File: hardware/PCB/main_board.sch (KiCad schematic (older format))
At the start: 0 parts

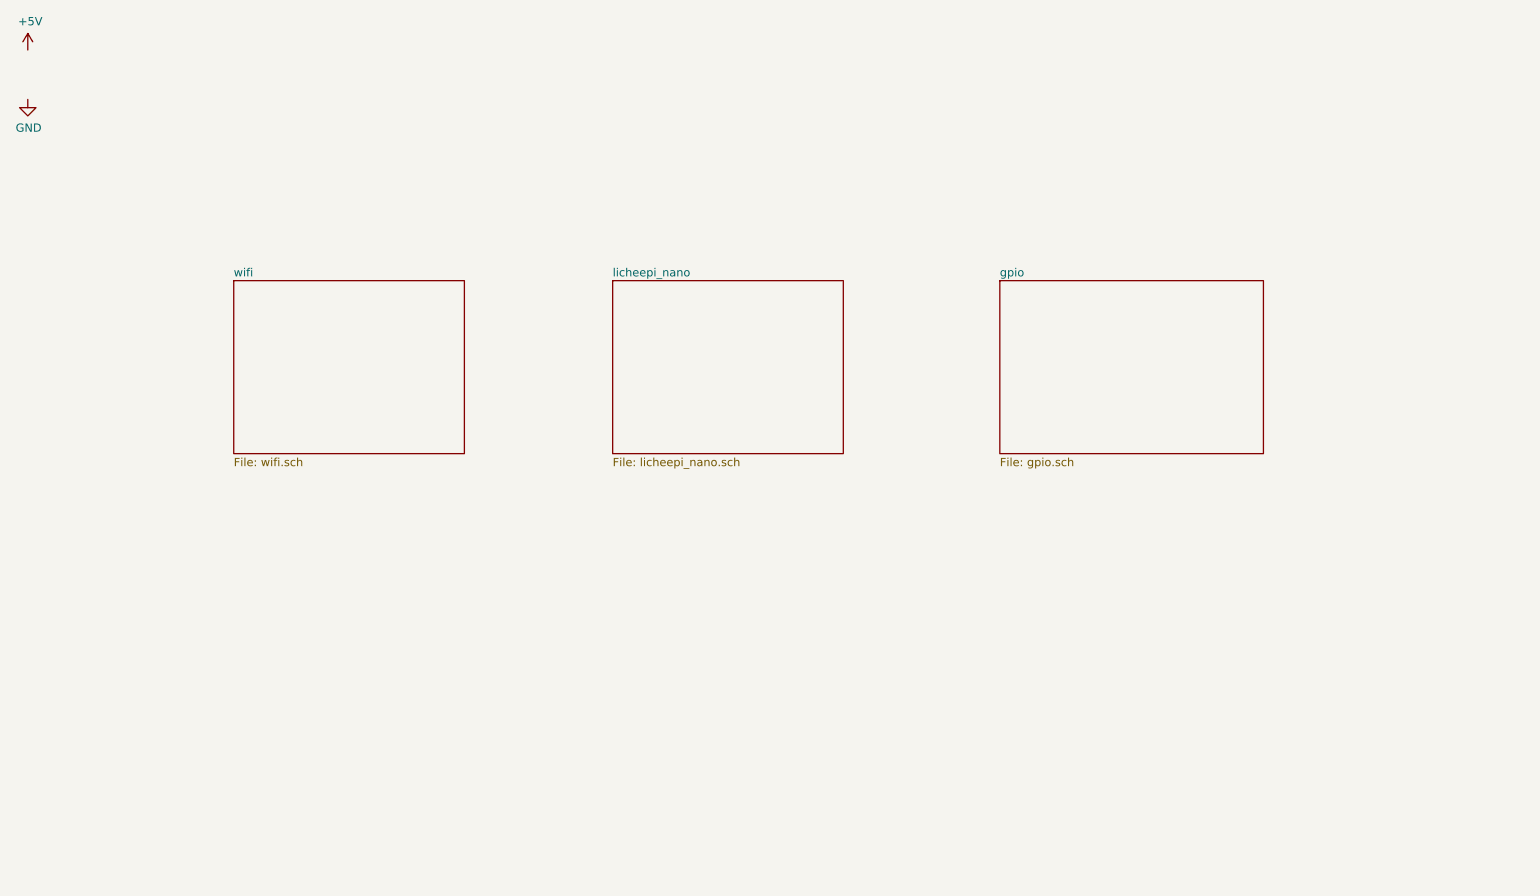
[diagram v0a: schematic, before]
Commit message: update pcb,
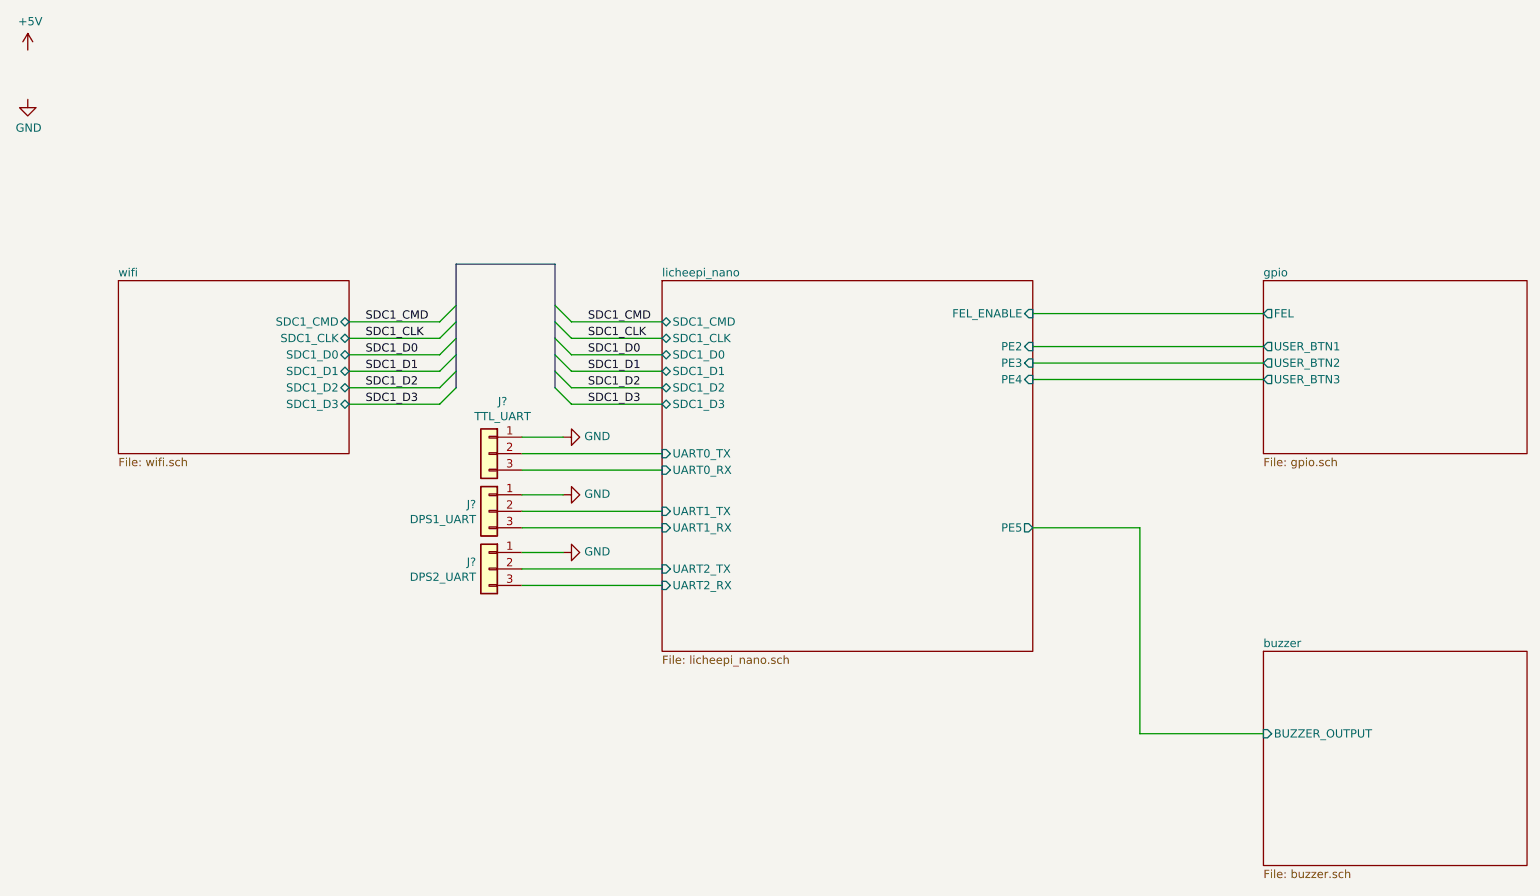
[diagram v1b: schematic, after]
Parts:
- added J?: TTL_UART, symbol Connector_Generic:Conn_01x03
- added J?: DPS1_UART, symbol Connector_Generic:Conn_01x03
- added J?: DPS2_UART, symbol Connector_Generic:Conn_01x03
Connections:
- net GND: now also J?.1 (Pin_1), J?.1 (Pin_1), J?.1 (Pin_1)
- new net licheepi_nano/UART0_RX: J?.3 (Pin_3)
- new net licheepi_nano/UART0_TX: J?.2 (Pin_2)
- new net licheepi_nano/UART1_RX: J?.3 (Pin_3)
- new net licheepi_nano/UART1_TX: J?.2 (Pin_2)
- new net licheepi_nano/UART2_RX: J?.3 (Pin_3)
- new net licheepi_nano/UART2_TX: J?.2 (Pin_2)
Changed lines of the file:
@@
 $Descr A4 11693 8268
 encoding utf-8
-Sheet 1 4
+Sheet 1 5
 Title ""
 Date ""
@@
 $EndDescr
 $Comp
-L customized_power:+5V #PWR?
+L customized_power:+5V #PWR0101
 U 1 1 5E8767E8
 P 950 1000
-F 0 "#PWR?" H 950 850 50  0001 C CNN
+F 0 "#PWR0101" H 950 850 50  0001 C CNN
 F 1 "+5V" H 965 1173 50  0000 C CNN
 F 2 "" H 950 1000 50  0001 C CNN
@@
 $EndComp
 $Comp
-L power:GND #PWR?
+L power:GND #PWR0102
 U 1 1 5E876DA9
 P 950 1300
-F 0 "#PWR?" H 950 1050 50  0001 C CNN
+F 0 "#PWR0102" H 950 1050 50  0001 C CNN
 F 1 "GND" H 955 1127 50  0000 C CNN
 F 2 "" H 950 1300 50  0001 C CNN
@@
 	1    0    0    -1
 $EndComp
-$Sheet
-S 4500 2400 1400 1050
+Entry Wire Line
+	3450 3150 3550 3050
+Entry Wire Line
+	3450 3050 3550 2950
+Entry Wire Line
+	3450 2950 3550 2850
+Entry Wire Line
+	3450 2850 3550 2750
+Entry Wire Line
+	3450 2750 3550 2650
+Entry Wire Line
+	3450 2650 3550 2550
+Wire Bus Line
+	3550 2300 4150 2300
+Entry Wire Line
+	4150 2550 4250 2650
+Entry Wire Line
+	4150 2650 4250 2750
+Entry Wire Line
+	4150 2750 4250 2850
+Entry Wire Line
+	4150 2850 4250 2950
+Entry Wire Line
+	4150 2950 4250 3050
+Entry Wire Line
+	4150 3050 4250 3150
+Wire Wire Line
+	4250 2650 4800 2650
+Wire Wire Line
+	4250 2750 4800 2750
+Wire Wire Line
+	4250 2850 4800 2850
+Wire Wire Line
+	4250 2950 4800 2950
+Wire Wire Line
+	4250 3050 4800 3050
+Wire Wire Line
+	4250 3150 4800 3150
+Wire Wire Line
+	2900 3150 3450 3150
+Wire Wire Line
+	2900 2650 3450 2650
+Wire Wire Line
+	2900 2750 3450 2750
+Wire Wire Line
+	2900 2850 3450 2850
+Wire Wire Line
+	2900 2950 3450 2950
+Wire Wire Line
+	2900 3050 3450 3050
+$Sheet
+S 1500 2400 1400 1050
+U 5E8B2717
+F0 "wifi" 50
+F1 "wifi.sch" 50
+F2 "SDC1_D2" B R 2900 3050 50
+F3 "SDC1_D1" B R 2900 2950 50
+F4 "SDC1_D0" B R 2900 2850 50
+F5 "SDC1_CLK" B R 2900 2750 50
+F6 "SDC1_CMD" B R 2900 2650 50
+F7 "SDC1_D3" B R 2900 3150 50
+$EndSheet
+Text Label 3000 2650 0    50   ~ 0
+SDC1_CMD
+Text Label 3000 2750 0    50   ~ 0
+SDC1_CLK
+Text Label 3000 2850 0    50   ~ 0
+SDC1_D0
+Text Label 3000 2950 0    50   ~ 0
+SDC1_D1
+Text Label 3000 3050 0    50   ~ 0
+SDC1_D2
+Text Label 3000 3150 0    50   ~ 0
+SDC1_D3
+Text Label 4350 2650 0    50   ~ 0
+SDC1_CMD
+Text Label 4350 2750 0    50   ~ 0
+SDC1_CLK
+Text Label 4350 2850 0    50   ~ 0
+SDC1_D0
+Text Label 4350 2950 0    50   ~ 0
+SDC1_D1
+Text Label 4350 3050 0    50   ~ 0
+SDC1_D2
+Text Label 4350 3150 0    50   ~ 0
+SDC1_D3
+$Sheet
+S 8450 4650 1600 1300
+U 5E91CDD8
+F0 "buzzer" 50
+F1 "buzzer.sch" 50
+F2 "BUZZER_OUTPUT" I L 8450 5150 50
+$EndSheet
+Wire Wire Line
+	7050 2600 8450 2600
+Wire Wire Line
+	7050 2800 8450 2800
+Wire Wire Line
+	7050 2900 8450 2900
+Wire Wire Line
+	7050 3000 8450 3000
+$Sheet
+S 8450 2400 1600 1050
+U 5E87CEF1
+F0 "gpio" 50
+F1 "gpio.sch" 50
+F2 "FEL" O L 8450 2600 50
+F3 "USER_BTN1" O L 8450 2800 50
+F4 "USER_BTN2" O L 8450 2900 50
+F5 "USER_BTN3" O L 8450 3000 50
+$EndSheet
+Wire Wire Line
+	7050 3900 7700 3900
+Wire Wire Line
+	7700 3900 7700 5150
+Wire Wire Line
+	7700 5150 8450 5150
+$Sheet
+S 4800 2400 2250 2250
 U 5E87A116
 F0 "licheepi_nano" 50
 F1 "licheepi_nano.sch" 50
-$EndSheet
-$Sheet
-S 6850 2400 1600 1050
-U 5E87CEF1
-F0 "gpio" 50
-F1 "gpio.sch" 50
-$EndSheet
-$Sheet
-S 2200 2400 1400 1050
-U 5E8B2717
-F0 "wifi" 50
-F1 "wifi.sch" 50
-$EndSheet
+F2 "SDC1_D2" B L 4800 3050 50
+F3 "SDC1_D1" B L 4800 2950 50
+F4 "SDC1_D0" B L 4800 2850 50
+F5 "SDC1_CLK" B L 4800 2750 50
+F6 "SDC1_CMD" B L 4800 2650 50
+F7 "SDC1_D3" B L 4800 3150 50
+F8 "FEL_ENABLE" I R 7050 2600 50
+F9 "PE2" I R 7050 2800 50
+F10 "PE3" I R 7050 2900 50
+F11 "PE4" I R 7050 3000 50
+F12 "PE5" O R 7050 3900 50
+F13 "UART0_TX" I L 4800 3450 50
+F14 "UART0_RX" I L 4800 3550 50
+F15 "UART1_TX" I L 4800 3800 50
+F16 "UART1_RX" I L 4800 3900 50
+F17 "UART2_RX" I L 4800 4250 50
+F18 "UART2_TX" I L 4800 4150 50
+$EndSheet
+$Comp
+L Connector_Generic:Conn_01x03 J?
+U 1 1 5E949A7D
+P 3750 3450
+F 0 "J?" H 3668 3767 50  0000 C CNN
+F 1 "TTL_UART" H 3668 3676 50  0000 C CNN
+F 2 "" H 3750 3450 50  0001 C CNN
+F 3 "~" H 3750 3450 50  0001 C CNN
+	1    3750 3450
+	-1   0    0    -1
+$EndComp
+$Comp
+L power:GND #PWR?
+U 1 1 5E94A27E
+P 4200 3350
+F 0 "#PWR?" H 4200 3100 50  0001 C CNN
+F 1 "GND" V 4205 3222 50  0000 R CNN
+F 2 "" H 4200 3350 50  0001 C CNN
+F 3 "" H 4200 3350 50  0001 C CNN
+	1    4200 3350
+	0    -1   -1   0
+$EndComp
+Wire Wire Line
+	3950 3350 4200 3350
+Wire Wire Line
+	3950 3450 4800 3450
+Wire Wire Line
+	3950 3550 4800 3550
+$Comp
+L Connector_Generic:Conn_01x03 J?
+U 1 1 5E94B27C
+P 3750 3800
+F 0 "J?" H 3829 3842 50  0000 L CNN
+F 1 "DPS1_UART" H 3829 3751 50  0000 L CNN
+F 2 "" H 3750 3800 50  0001 C CNN
+F 3 "~" H 3750 3800 50  0001 C CNN
+	1    3750 3800
+	-1   0    0    -1
+$EndComp
+$Comp
+L power:GND #PWR?
+U 1 1 5E94B286
+P 4200 3700
+F 0 "#PWR?" H 4200 3450 50  0001 C CNN
+F 1 "GND" V 4205 3572 50  0000 R CNN
+F 2 "" H 4200 3700 50  0001 C CNN
+F 3 "" H 4200 3700 50  0001 C CNN
+	1    4200 3700
+	0    -1   -1   0
+$EndComp
+Wire Wire Line
+	3950 3700 4200 3700
+Wire Wire Line
+	3950 3800 4800 3800
+Wire Wire Line
+	3950 3900 4800 3900
+$Comp
+L Connector_Generic:Conn_01x03 J?
+U 1 1 5E94C724
+P 3750 4150
+F 0 "J?" H 3829 4192 50  0000 L CNN
+F 1 "DPS2_UART" H 3829 4101 50  0000 L CNN
+F 2 "" H 3750 4150 50  0001 C CNN
+F 3 "~" H 3750 4150 50  0001 C CNN
+	1    3750 4150
+	-1   0    0    -1
+$EndComp
+$Comp
+L power:GND #PWR?
+U 1 1 5E94C72E
+P 4200 4050
+F 0 "#PWR?" H 4200 3800 50  0001 C CNN
+F 1 "GND" V 4205 3922 50  0000 R CNN
+F 2 "" H 4200 4050 50  0001 C CNN
+F 3 "" H 4200 4050 50  0001 C CNN
+	1    4200 4050
+	0    -1   -1   0
+$EndComp
+Wire Wire Line
+	3950 4050 4200 4050
+Wire Wire Line
+	3950 4150 4800 4150
+Wire Wire Line
+	3950 4250 4800 4250
+Wire Bus Line
+	3550 2300 3550 3050
+Wire Bus Line
+	4150 2300 4150 3050
 $EndSCHEMATC
